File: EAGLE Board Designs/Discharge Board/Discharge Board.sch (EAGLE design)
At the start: 7 parts, among them J1 CONNECTOR-2_MICROFIT_SMD_RIGH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, J2 CONNECTOR-2_MICROFIT_SMD_RIGH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, K1 RELAY_SPST_NC_POLARIZED_D_24

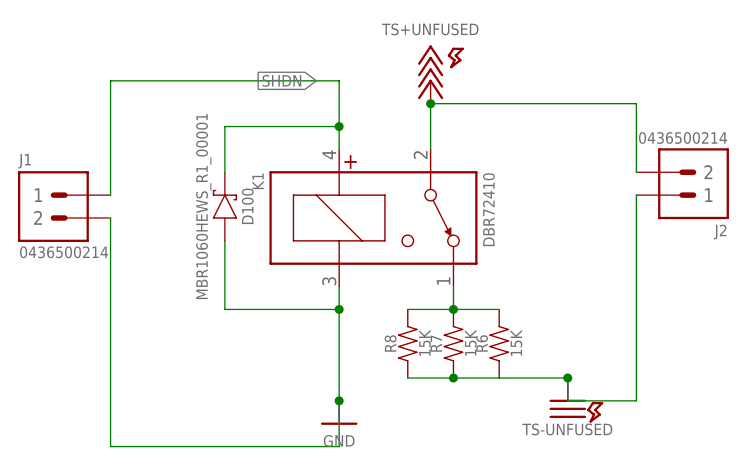
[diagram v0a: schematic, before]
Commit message: made components fit better?
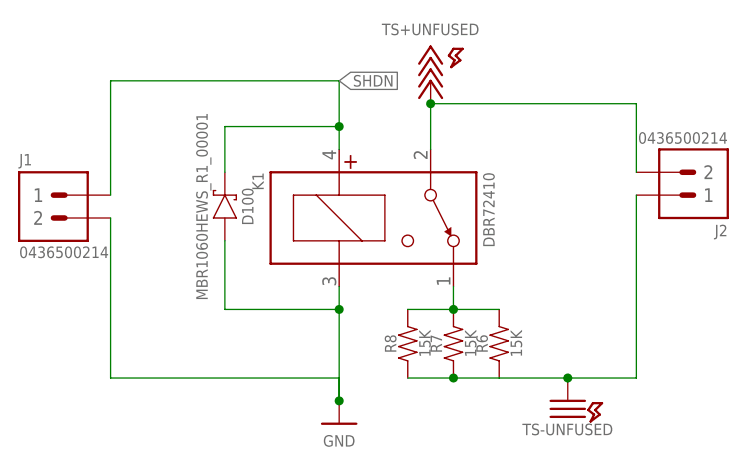
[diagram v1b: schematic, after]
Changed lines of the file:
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@@
 <pinref part="K1" gate="G$1" pin="COIL-"/>
 <pinref part="J1" gate="G$1" pin="2"/>
-<wire x1="-2.54" y1="30.48" x2="-2.54" y2="5.08" width="0.1524" layer="91"/>
-<wire x1="-2.54" y1="5.08" x2="22.86" y2="5.08" width="0.1524" layer="91"/>
-<wire x1="22.86" y1="5.08" x2="22.86" y2="10.16" width="0.1524" layer="91"/>
+<wire x1="-2.54" y1="30.48" x2="-2.54" y2="12.7" width="0.1524" layer="91"/>
+<wire x1="-2.54" y1="12.7" x2="22.86" y2="12.7" width="0.1524" layer="91"/>
+<wire x1="22.86" y1="12.7" x2="22.86" y2="10.16" width="0.1524" layer="91"/>
 <junction x="22.86" y="10.16"/>
 </segment>
@@
 <wire x1="22.86" y1="40.64" x2="22.86" y2="38.1" width="0.1524" layer="91"/>
 <junction x="22.86" y="40.64"/>
-<label x="20.32" y="45.72" size="1.27" layer="95" rot="MR0" xref="yes"/>
+<label x="22.86" y="45.72" size="1.27" layer="95" rot="MR180" xref="yes"/>
 <wire x1="22.86" y1="40.64" x2="22.86" y2="45.72" width="0.1524" layer="91"/>
-<wire x1="22.86" y1="45.72" x2="20.32" y2="45.72" width="0.1524" layer="91"/>
 <pinref part="K1" gate="G$1" pin="COIL+"/>
 <pinref part="J1" gate="G$1" pin="1"/>
 <wire x1="-2.54" y1="33.02" x2="-2.54" y2="45.72" width="0.1524" layer="91"/>
-<wire x1="-2.54" y1="45.72" x2="20.32" y2="45.72" width="0.1524" layer="91"/>
+<wire x1="-2.54" y1="45.72" x2="22.86" y2="45.72" width="0.1524" layer="91"/>
 </segment>
 </net>
@@
 <pinref part="K1" gate="G$1" pin="CONTACT1"/>
 <pinref part="J2" gate="G$1" pin="2"/>
-<wire x1="55.88" y1="35.56" x2="55.88" y2="43.18" width="0.1524" layer="91"/>
-<wire x1="55.88" y1="43.18" x2="33.02" y2="43.18" width="0.1524" layer="91"/>
+<wire x1="55.88" y1="35.56" x2="55.88" y2="43.18" width="0.6096" layer="91"/>
+<wire x1="55.88" y1="43.18" x2="33.02" y2="43.18" width="0.6096" layer="91"/>
 <junction x="33.02" y="43.18"/>
 </segment>
@@
 <wire x1="40.64" y1="12.7" x2="48.26" y2="12.7" width="0.6096" layer="91"/>
 <pinref part="J2" gate="G$1" pin="1"/>
-<wire x1="55.88" y1="33.02" x2="55.88" y2="10.16" width="0.1524" layer="91"/>
-<wire x1="55.88" y1="10.16" x2="48.26" y2="10.16" width="0.1524" layer="91"/>
-<wire x1="48.26" y1="10.16" x2="48.26" y2="12.7" width="0.1524" layer="91"/>
+<wire x1="55.88" y1="33.02" x2="55.88" y2="12.7" width="0.6096" layer="91"/>
+<wire x1="55.88" y1="12.7" x2="48.26" y2="12.7" width="0.6096" layer="91"/>
 <junction x="48.26" y="12.7"/>
 </segment>
